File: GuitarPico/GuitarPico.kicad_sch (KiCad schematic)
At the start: 132 parts, among them J1 INPUT, J2 INPUT, J3 OUTPUT, J4 OUTPUT, J5 Barrel_Jack_Switch, J6 VGA, J8 INPUT, J9 INPUT, Q1 2N3904, Q2 2N3904, Q3 2N3904, SW1 SW_Push, SW2 SW_Push, SW3 SW_Push, SW4 SW_Push, SW5 SW_Push, U1 LM358, U2 LM358, U3 Pico, U4 LM7805_TO220, U5 TL431LP, U6 4051

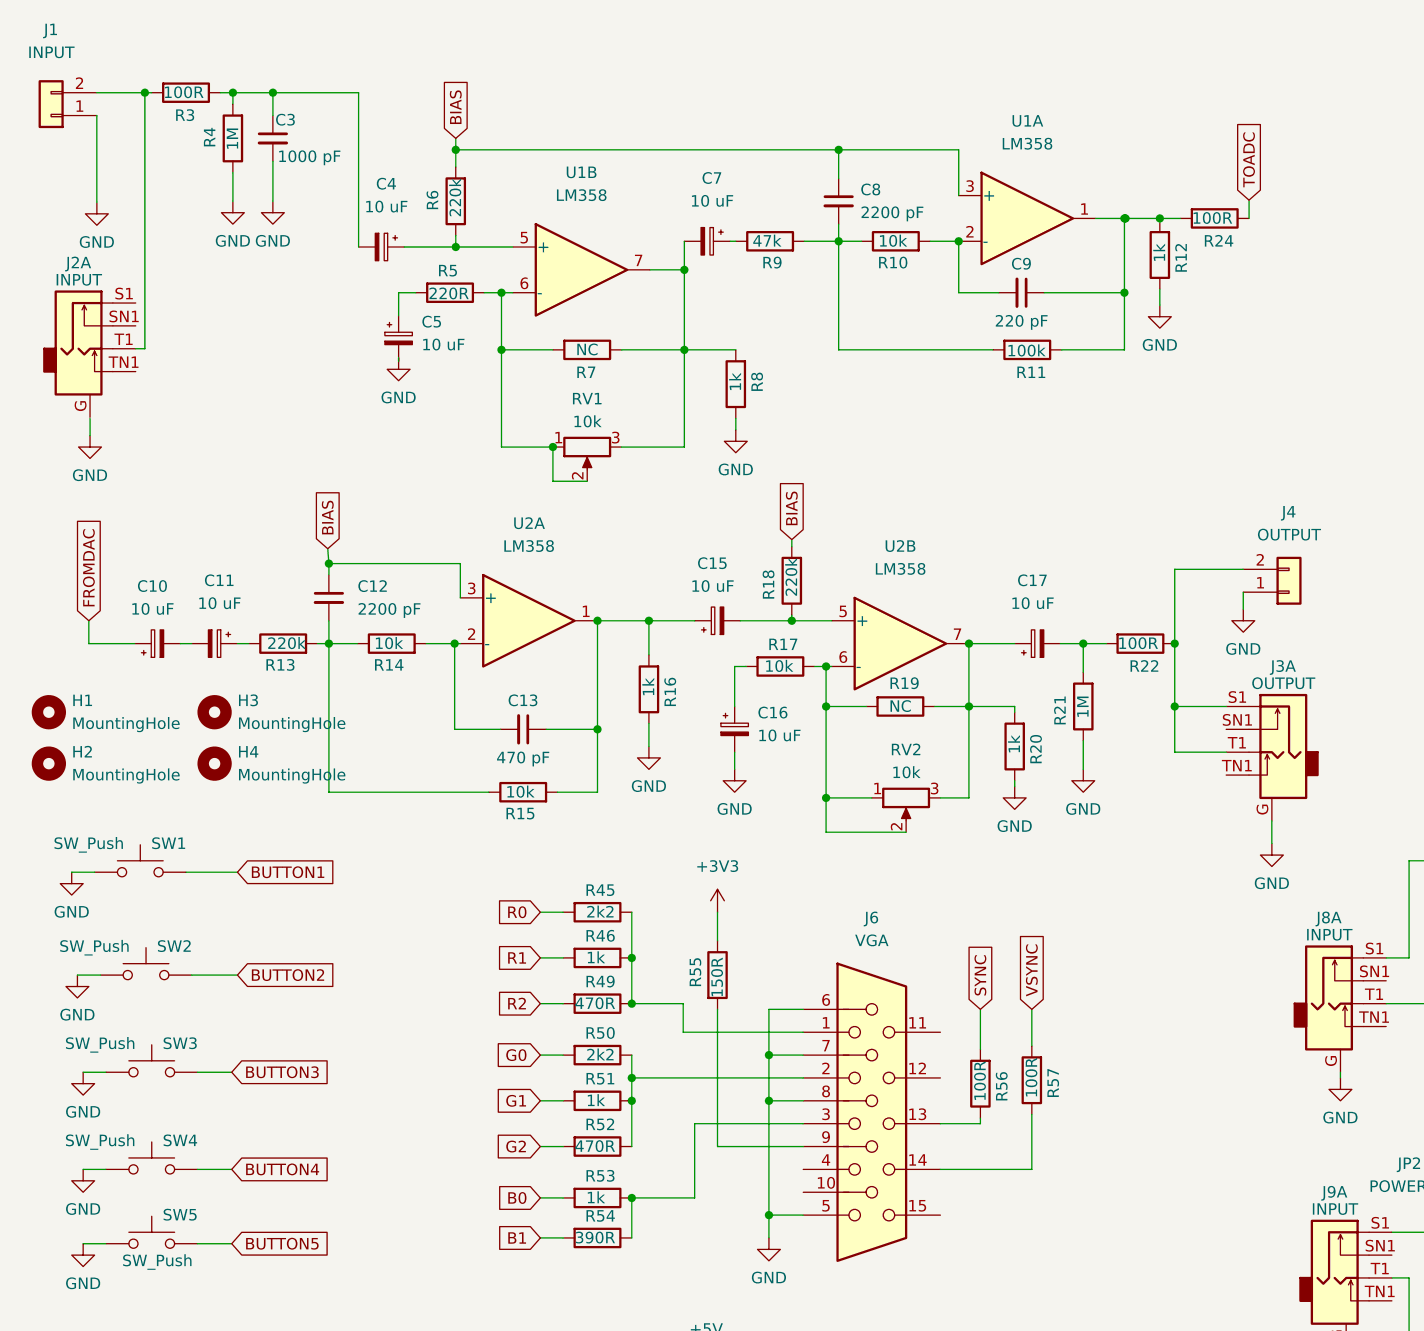
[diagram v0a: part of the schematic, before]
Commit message: Minor code fixes
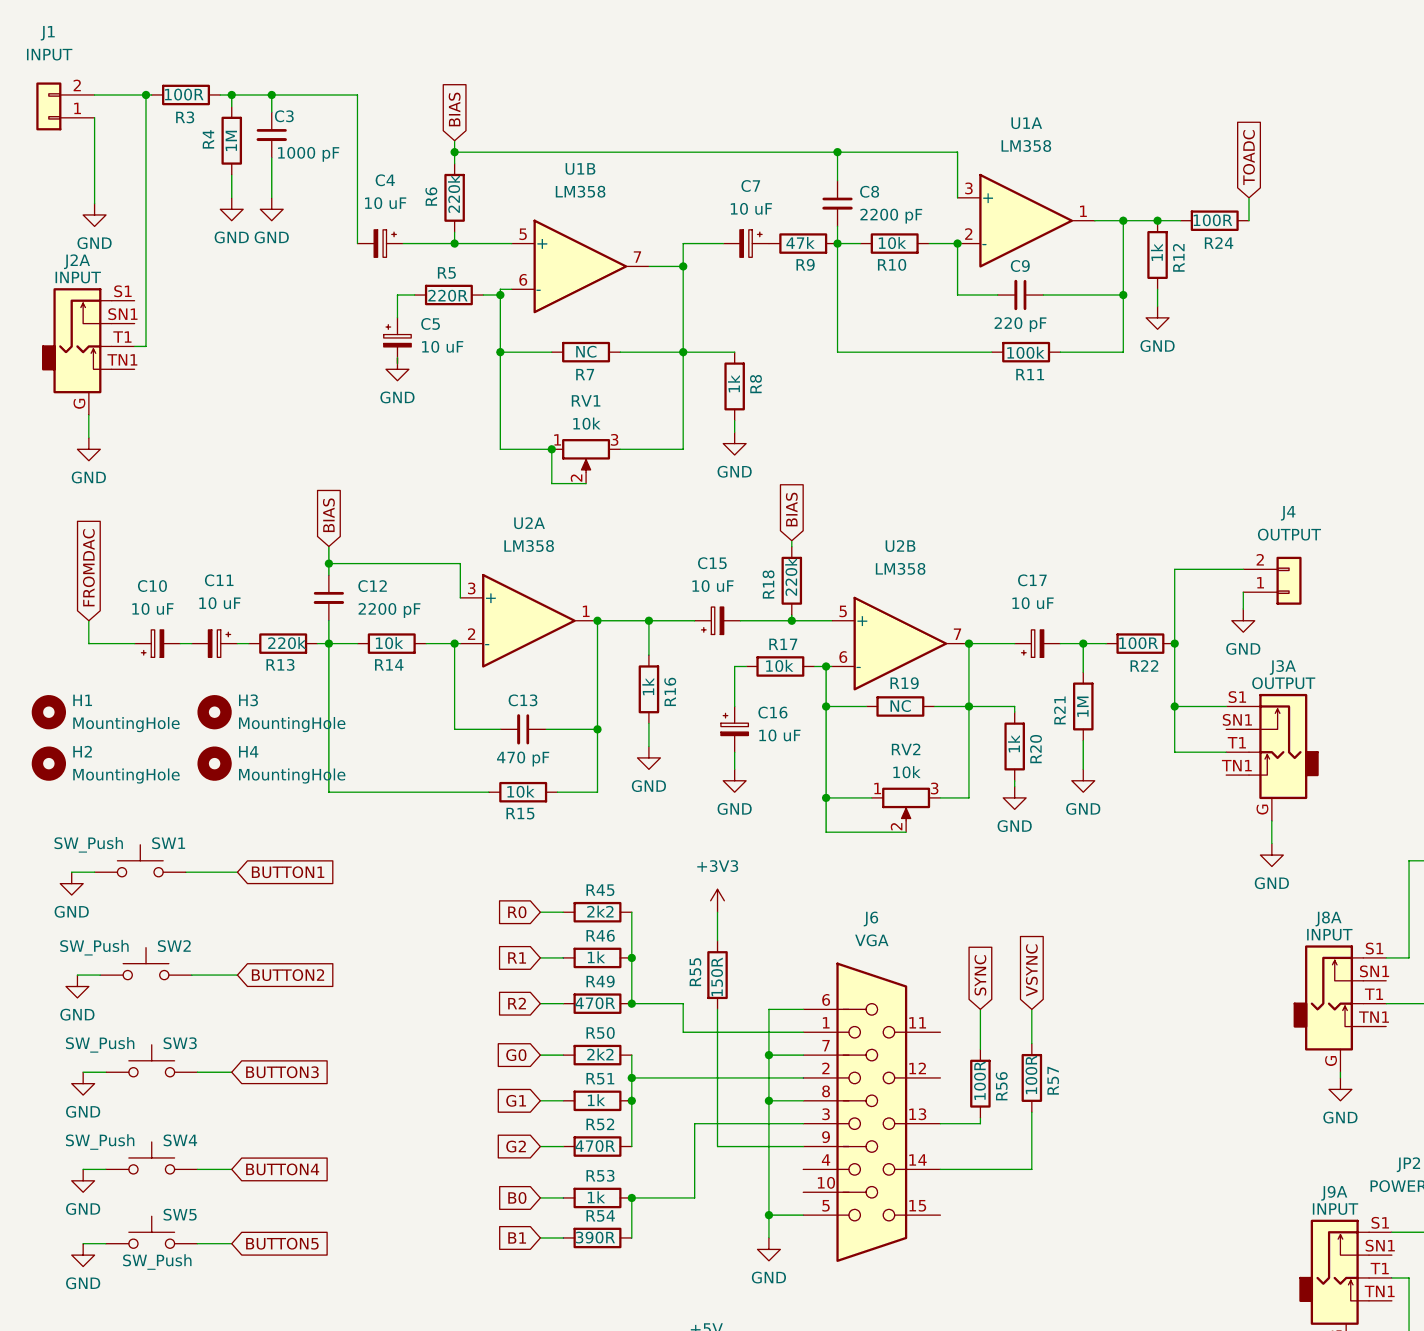
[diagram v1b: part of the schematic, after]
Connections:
- net GND: now also J2.G
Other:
- moved on the sheet: C7, R9
